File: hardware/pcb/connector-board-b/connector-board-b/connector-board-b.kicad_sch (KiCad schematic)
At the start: 4 parts, among them J1 DE9_Pins, J3 Conn_01x02, J4 Conn_01x02, J5 8-215570-0

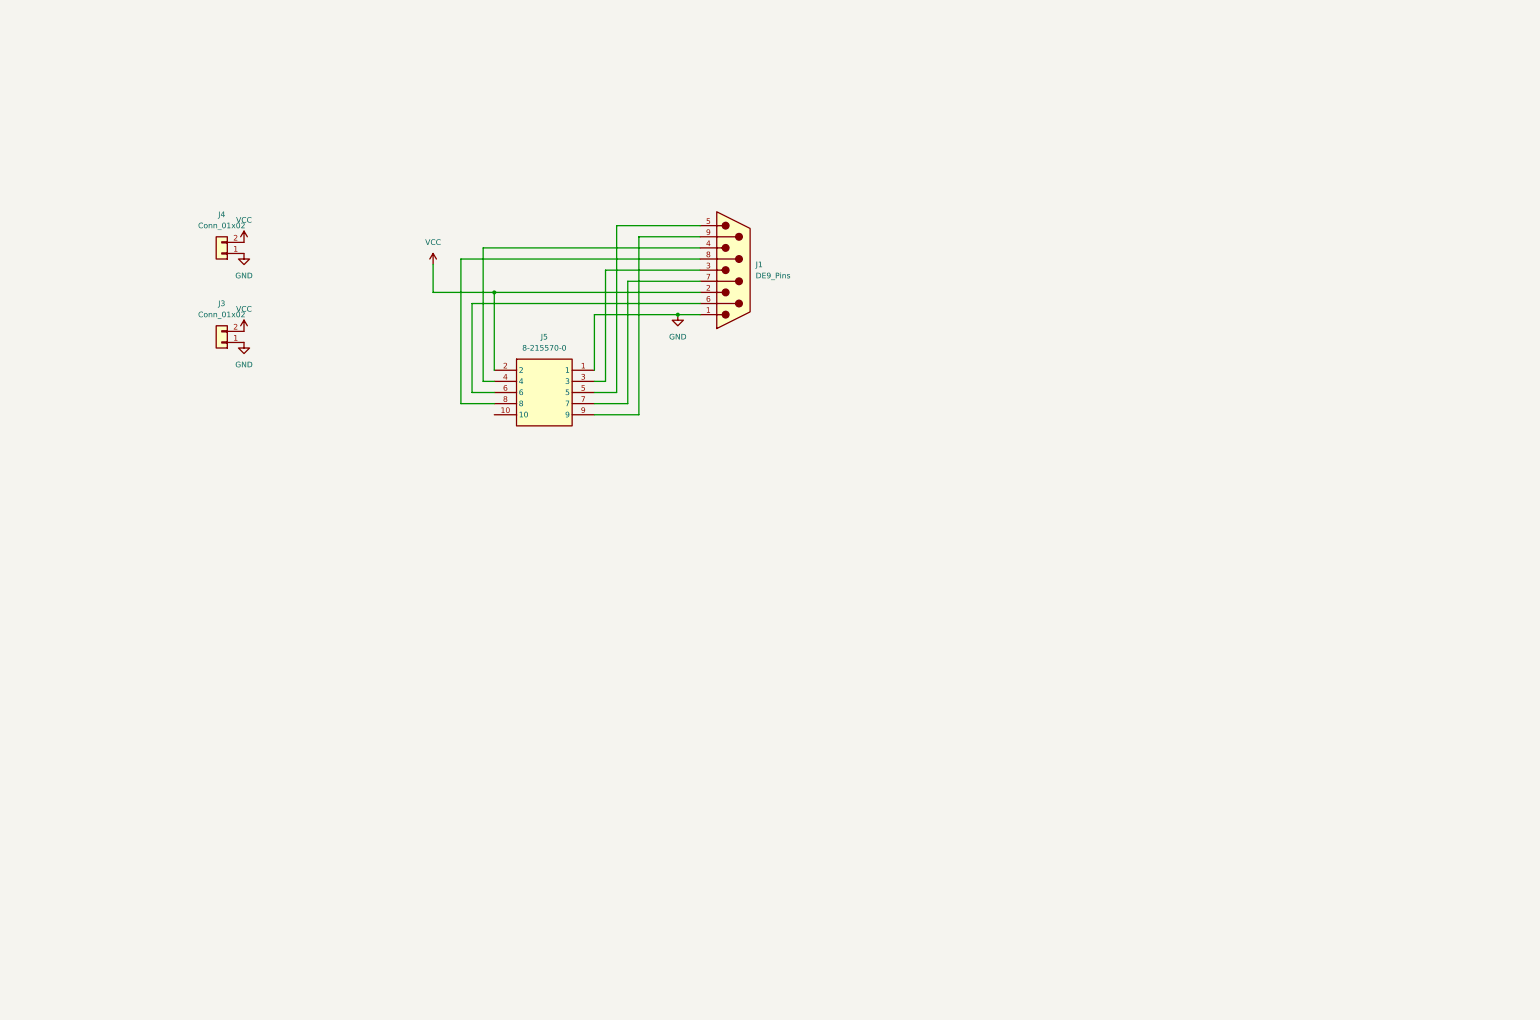
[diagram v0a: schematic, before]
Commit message: Updated Connectorboard B to rev. 1.1
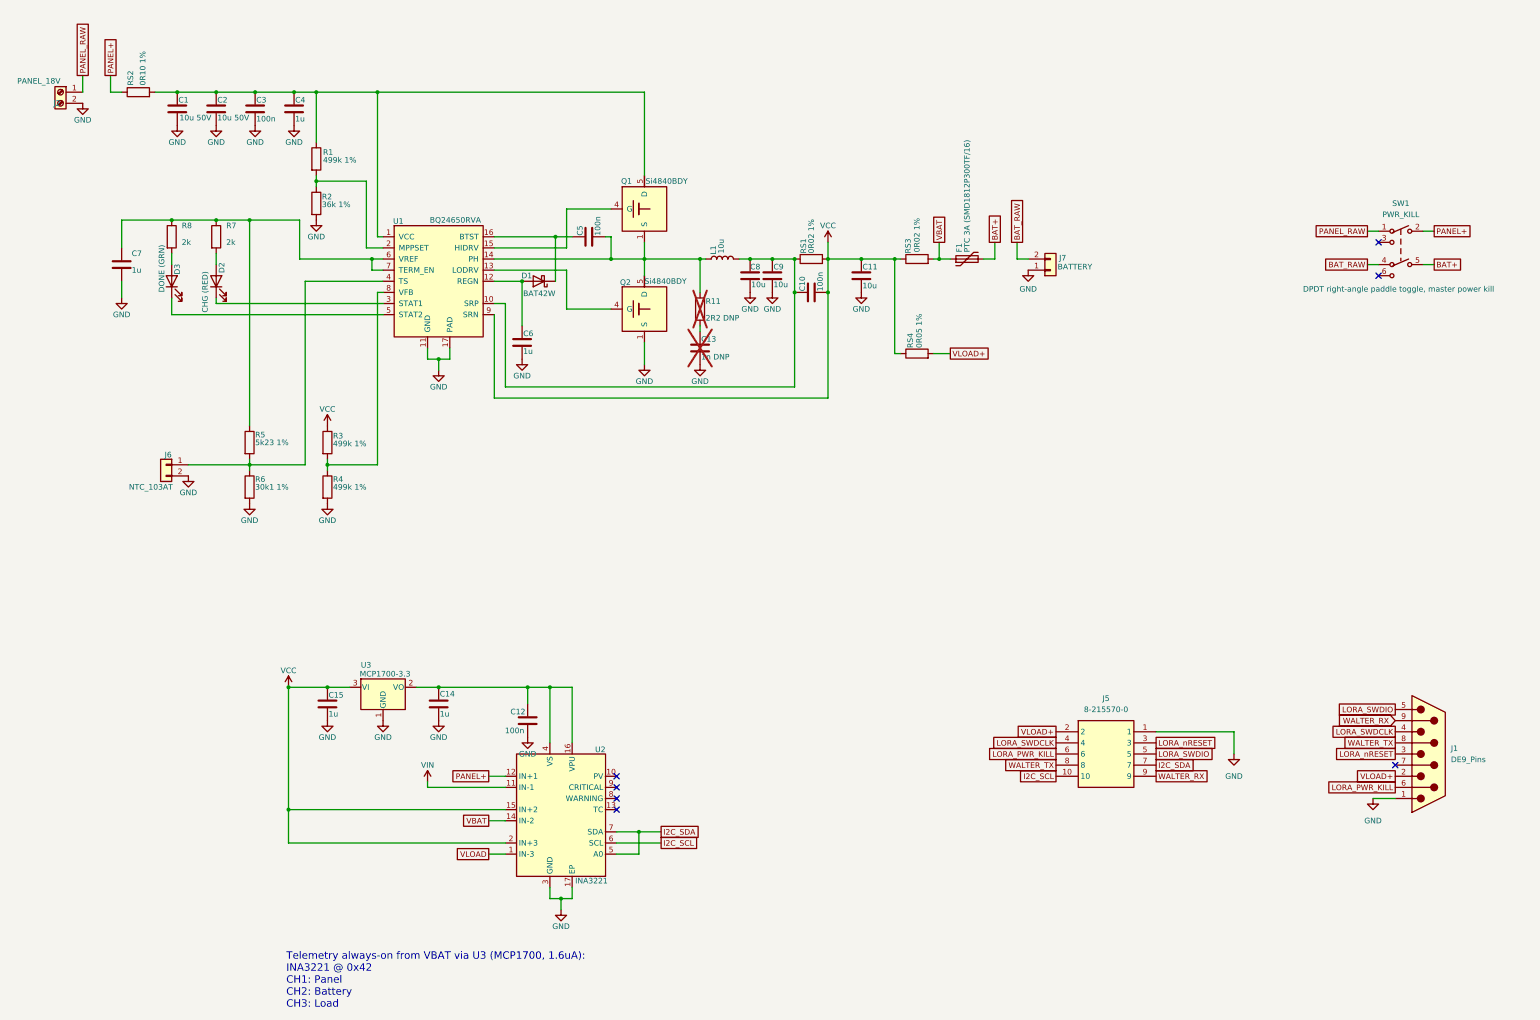
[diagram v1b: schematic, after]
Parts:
- removed J3: Conn_01x02, TerminalBlock:TerminalBlock_MaiXu_MX126-5.0-02P_1x02_P5.00mm, symbol Connector_Generic:Conn_01x02
- removed J4: Conn_01x02, Connector_JST:JST_EH_B2B-EH-A_1x02_P2.50mm_Vertical, symbol Connector_Generic:Conn_01x02
- added C1, C2: 10u 50V, Capacitor_SMD:C_1210_3225Metric, symbol Device:C
- added C10, C12, C3, C5: 100n, Capacitor_SMD:C_0805_2012Metric, symbol Device:C
- added C11, C8, C9: 10u, Capacitor_SMD:C_1206_3216Metric, symbol Device:C
- added C13: 1n DNP, Capacitor_SMD:C_0805_2012Metric, symbol Device:C
- added C14, C15, C4, C6, C7: 1u, Capacitor_SMD:C_0805_2012Metric, symbol Device:C
- added D1: BAT42W, Diode_SMD:D_SOD-123, symbol Device:D_Schottky
- added D2: CHG (RED), LED_SMD:LED_0805_2012Metric, symbol Device:LED
- added D3: DONE (GRN), LED_SMD:LED_0805_2012Metric, symbol Device:LED
- added F1: PTC 3A (SMD1812P300TF/16), Fuse:Fuse_1812_4532Metric, symbol Device:Polyfuse
- added J2: PANEL_18V, TerminalBlock:TerminalBlock_MaiXu_MX126-5.0-02P_1x02_P5.00mm, symbol Connector:Screw_Terminal_01x02
- added J6: NTC_103AT, Connector_JST:JST_PH_B2B-PH-K_1x02_P2.00mm_Vertical, symbol Connector_Generic:Conn_01x02
- added J7: BATTERY, Connector_JST:JST_EH_B2B-EH-A_1x02_P2.50mm_Vertical, symbol Connector_Generic:Conn_01x02
- added L1: 10u, Inductor_SMD:L_Vishay_IHLP-4040, symbol Device:L
- added Q1, Q2: Si4840BDY, Package_SO:SOIC-8_3.9x4.9mm_P1.27mm, symbol solar_charger:NMOS_SOIC8
- added R1, R3, R4: 499k 1%, Resistor_SMD:R_0805_2012Metric, symbol Device:R
- added R11: 2R2 DNP, Resistor_SMD:R_0805_2012Metric, symbol Device:R
- added R2: 36k 1%, Resistor_SMD:R_0805_2012Metric, symbol Device:R
- added R5: 5k23 1%, Resistor_SMD:R_0805_2012Metric, symbol Device:R
- added R6: 30k1 1%, Resistor_SMD:R_0805_2012Metric, symbol Device:R
- added R7, R8: 2k, Resistor_SMD:R_0805_2012Metric, symbol Device:R
- added RS1, RS3: 0R02 1%, Resistor_SMD:R_1206_3216Metric, symbol Device:R
- added RS2: 0R10 1%, Resistor_SMD:R_1206_3216Metric, symbol Device:R
- added RS4: 0R05 1%, Resistor_SMD:R_1206_3216Metric, symbol Device:R
- added SW1: PWR_KILL, connector-board-b:SW_Toggle_CAX_MTS202C3D1_RightAngle, symbol adapter:SW_DPDT
- added U1: BQ24650RVA, solar_charger:Texas_RVA0016A_VQFN-16-1EP_3.5x3.5mm_P0.5mm_EP2.1x2.1mm, symbol solar_charger:BQ24650RVA
- added U2: INA3221, Package_DFN_QFN:Texas_RGV0016A_VQFN-16-1EP_4x4mm_P0.65mm_EP2.1x2.1mm, symbol Power_Management:INA3221
- added U3: MCP1700-3.3, Package_TO_SOT_SMD:SOT-23, symbol Regulator_Linear:MCP1700x-300xxTT
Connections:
- net GND: now also C1.2, C11.2, C12.2, C13.2, C14.2, C15.2, C2.2, C3.2, C4.2, C6.2, C7.2, C8.2, C9.2, J2.2 (Pin_2), J6.2 (Pin_2), J7.1 (Pin_1), Q2.1 (S), Q2.2 (S), Q2.3 (S), R2.2, R4.2, R6.2, U1.11 (GND), U1.17 (PAD), U2.17 (EP), U2.3 (GND), U3.1 (GND)
- net VCC: now also C10.2, C11.1, C15.1, R3.1, RS1.2, RS3.1, RS4.1, U1.9 (SRN), U2.15 (IN+2), U2.2 (IN+3), U3.3 (VI); no longer J1.2, J5.2
- net LORA_nRESET: now reaches J1.3, J5.3
- net LORA_SWDCLK: now reaches J1.4, J5.4
- net LORA_SWDIO: now reaches J1.5, J5.5
- net LORA_PWR_KILL: now reaches J1.6, J5.6
- net at J1.7: no longer J5.7
- net WALTER_TX: now reaches J1.8, J5.8
- net WALTER_RX: now reaches J1.9, J5.9
- net I2C_SCL: now reaches J5.10
- net I2C_SCL: now also U2.6 (SCL)
- new net: C12.1, C14.1, U2.16 (VPU), U2.4 (VS), U3.2 (VO)
- new net: C10.1, C8.1, C9.1, L1.2, RS1.1, U1.10 (SRP)
- new net: D3.1 (K), U1.5 (STAT2)
- new net: D3.2 (A), R8.2
- new net: C1.1, C2.1, C3.1, C4.1, Q1.5 (D), Q1.6 (D), Q1.7 (D), Q1.8 (D), R1.1, RS2.2, U1.1 (VCC)
- new net: J6.1 (Pin_1), R5.2, R6.1, U1.4 (TS)
- new net: C7.1, R5.1, R7.1, R8.1, U1.6 (VREF), U1.7 (TERM_EN)
- new net: D2.2 (A), R7.2
- new net: R3.2, R4.1, U1.8 (VFB)
- new net: C5.1, D1.1 (K), U1.16 (BTST)
- new net: C5.2, L1.1, Q1.1 (S), Q1.2 (S), Q1.3 (S), Q2.5 (D), Q2.6 (D), Q2.7 (D), Q2.8 (D), R11.1, U1.14 (PH)
- new net: C6.1, D1.2 (A), U1.12 (REGN)
- new net: Q2.4 (G), U1.13 (LODRV)
- new net: Q1.4 (G), U1.15 (HIDRV)
- new net: R1.2, R2.1, U1.2 (MPPSET)
- new net: D2.1 (K), U1.3 (STAT1)
- new net: C13.1, R11.2
- new net BAT+: F1.2, SW1.5 (COM2)
- new net BAT_RAW: J7.2 (Pin_2), SW1.4 (A2)
- new net I2C_SDA: J5.7, U2.5 (A0), U2.7 (SDA)
- new net PANEL+: RS2.1, SW1.2 (COM1), U2.12 (IN+1)
- new net PANEL_RAW: J2.1 (Pin_1), SW1.1 (A1)
- new net VBAT: F1.1, RS3.2, U2.14 (IN-2)
- new net VIN: U2.11 (IN-1)
- new net VLOAD: U2.1 (IN-3)
- new net VLOAD+: J1.2, J5.2, RS4.2
- no-connect marks 0 -> 7
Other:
- note added: "Telemetry always-on from VBAT via U3 (MCP1700, 1.6uA): INA3221 @ 0x42 CH1: Panel CH2: Battery CH3: Load"
- moved on the sheet: J1, J5
